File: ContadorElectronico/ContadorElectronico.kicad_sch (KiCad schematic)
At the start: 26 parts, among them J1 Screw_Terminal_01x02, J2 Screw_Terminal_01x02, SW1 MODE, SW2 INC, SW3 DEC, U2 LM7809_TO220, U4 LM358, U5 4N35, U6 4N35

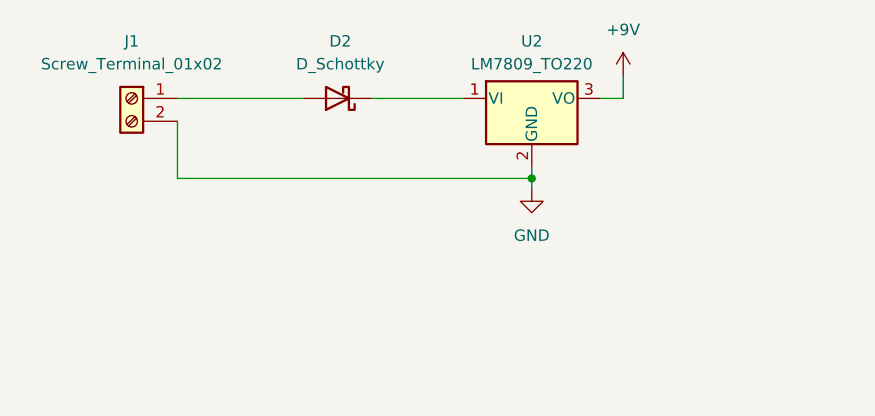
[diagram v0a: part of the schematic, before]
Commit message: xd
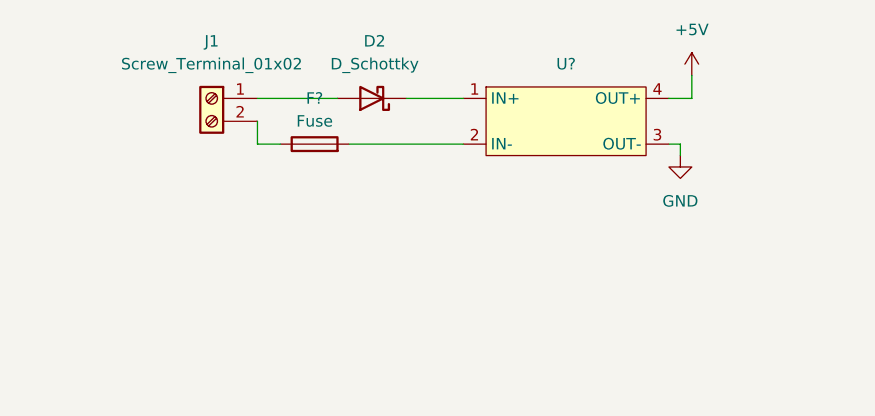
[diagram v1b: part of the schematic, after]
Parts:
- removed U2: LM7809_TO220, Package_TO_SOT_THT:TO-220-3_Vertical, symbol Regulator_Linear:LM7809_TO220
- added F?: Fuse, symbol Device:Fuse
- added U?: ~, symbol Custom:LM2596_MODULE
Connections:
- net +5V: now also U?.4 (OUT+)
- net GND: now also U?.3 (OUT-); no longer J1.2 (Pin_2)
- net at D2.1 (K): now also U?.1 (IN+)
- new net: F?.2, U?.2 (IN-)
- new net: F?.1, J1.2 (Pin_2)
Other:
- moved on the sheet: D2, J1
